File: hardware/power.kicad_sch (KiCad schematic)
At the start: 48 parts, among them J1 USB4085-GF-A, J2 Batteries, J3 Conn_01x02, J4 Conn_01x02, J5 Conn_01x02, J6 Conn_01x02, Q1 PMOS, Q2 PMOS, Q3 PMOS, U1 USBLC6-2SC6, U2 TLV76733DGNR

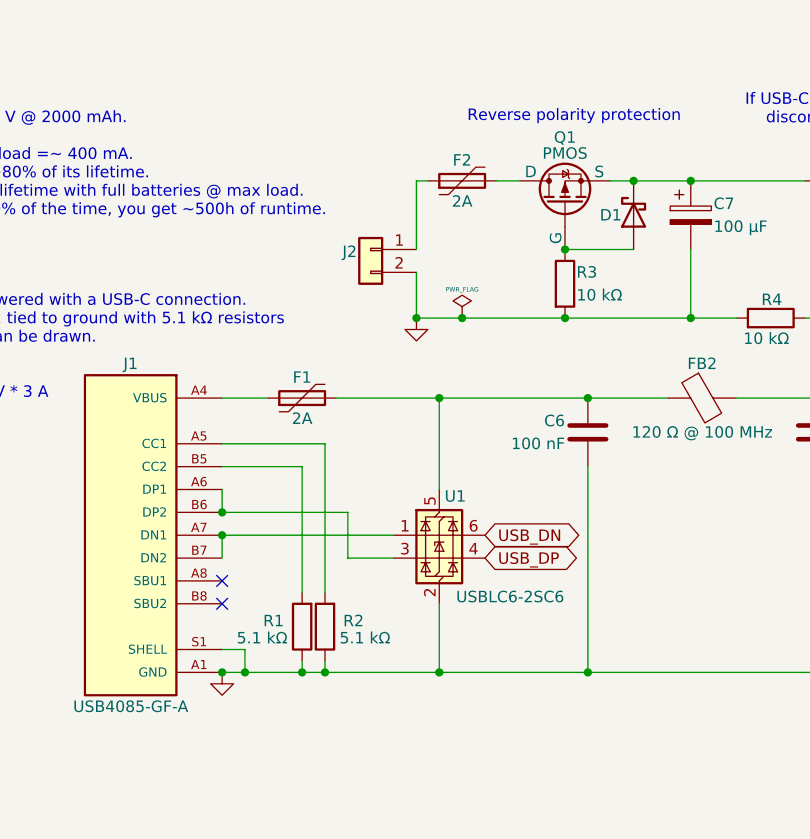
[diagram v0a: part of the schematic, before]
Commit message: HW: Layout power section
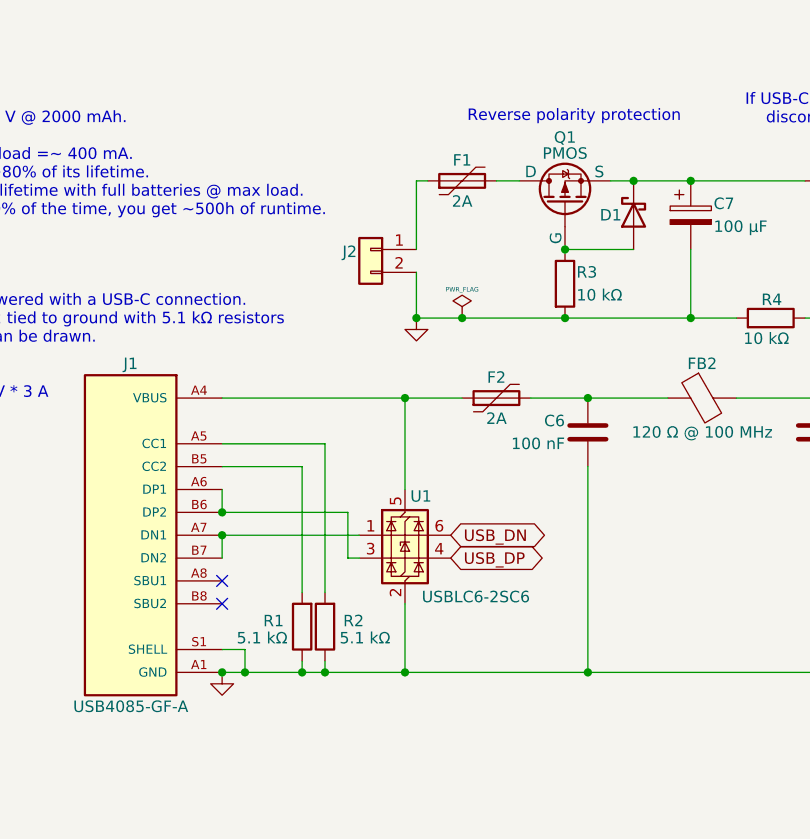
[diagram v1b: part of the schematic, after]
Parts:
- renumbered F2 to F1, F1 to F2
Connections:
- net at F2.1, J1.A4 (VBUS), J1.A9 (VBUS)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: now also U1.5 (VBUS)
- net at C6.1, F2.2, FB2.1: no longer U1.5 (VBUS)
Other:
- moved on the sheet: F2, U1
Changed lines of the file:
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@@
 	)
 	(junction
+		(at 116.84 66.04)
+		(diameter 0)
+		(color 0 0 0 0)
+	)
+	(junction
 		(at 116.84 96.52)
 		(diameter 0)
@@
 	)
 	(junction
-		(at 116.84 66.04)
+		(at 96.52 66.04)
 		(diameter 0)
 		(color 0 0 0 0)
@@
 	)
 	(junction
-		(at 100.33 66.04)
-		(diameter 0)
-		(color 0 0 0 0)
-	)
-	(junction
 		(at 170.18 88.9)
 		(diameter 0)
@@
 	)
 	(junction
-		(at 100.33 96.52)
-		(diameter 0)
-		(color 0 0 0 0)
-	)
-	(junction
 		(at 91.44 185.42)
 		(diameter 0)
@@
 	)
 	(junction
+		(at 96.52 96.52)
+		(diameter 0)
+		(color 0 0 0 0)
+	)
+	(junction
 		(at 204.47 148.59)
 		(diameter 0)
@@
 	(wire
 		(pts
-			(xy 100.33 66.04) (xy 100.33 76.2)
+			(xy 96.52 66.04) (xy 96.52 76.2)
 		)
 		(stroke
@@
 	(wire
 		(pts
-			(xy 100.33 66.04) (xy 116.84 66.04)
+			(xy 229.87 41.91) (xy 231.14 41.91)
 		)
 		(stroke
@@
 	(wire
 		(pts
-			(xy 229.87 41.91) (xy 231.14 41.91)
+			(xy 80.01 193.04) (xy 91.44 193.04)
 		)
 		(stroke
@@
 	(wire
 		(pts
-			(xy 80.01 193.04) (xy 91.44 193.04)
+			(xy 78.74 96.52) (xy 85.09 96.52)
 		)
 		(stroke
@@
 	(wire
 		(pts
-			(xy 78.74 96.52) (xy 85.09 96.52)
+			(xy 163.83 148.59) (xy 172.72 148.59)
 		)
 		(stroke
@@
 	(wire
 		(pts
-			(xy 163.83 148.59) (xy 172.72 148.59)
+			(xy 68.58 185.42) (xy 80.01 185.42)
 		)
 		(stroke
@@
 	(wire
 		(pts
-			(xy 68.58 185.42) (xy 80.01 185.42)
+			(xy 96.52 66.04) (xy 102.87 66.04)
 		)
 		(stroke
@@
 	(wire
 		(pts
-			(xy 100.33 96.52) (xy 116.84 96.52)
+			(xy 146.05 49.53) (xy 146.05 57.15)
 		)
 		(stroke
@@
 	(wire
 		(pts
-			(xy 146.05 49.53) (xy 146.05 57.15)
+			(xy 96.52 96.52) (xy 116.84 96.52)
 		)
 		(stroke
@@
 	(wire
 		(pts
-			(xy 88.9 66.04) (xy 100.33 66.04)
+			(xy 229.87 66.04) (xy 238.76 66.04)
 		)
 		(stroke
@@
 	(wire
 		(pts
-			(xy 229.87 66.04) (xy 238.76 66.04)
+			(xy 194.31 130.81) (xy 207.01 130.81)
 		)
 		(stroke
@@
 	(wire
 		(pts
-			(xy 194.31 130.81) (xy 207.01 130.81)
+			(xy 76.2 81.28) (xy 91.44 81.28)
 		)
 		(stroke
@@
 	(wire
 		(pts
-			(xy 76.2 81.28) (xy 95.25 81.28)
+			(xy 128.27 57.15) (xy 133.35 57.15)
 		)
 		(stroke
@@
 	(wire
 		(pts
-			(xy 128.27 57.15) (xy 133.35 57.15)
+			(xy 168.91 123.19) (xy 181.61 123.19)
 		)
 		(stroke
@@
 	(wire
 		(pts
-			(xy 168.91 123.19) (xy 181.61 123.19)
+			(xy 182.88 96.52) (xy 191.77 96.52)
 		)
 		(stroke
@@
 	(wire
 		(pts
-			(xy 182.88 96.52) (xy 191.77 96.52)
+			(xy 102.87 57.15) (xy 114.3 57.15)
 		)
 		(stroke
@@
 	(wire
 		(pts
-			(xy 102.87 57.15) (xy 114.3 57.15)
+			(xy 96.52 88.9) (xy 96.52 96.52)
 		)
 		(stroke
@@
 	(wire
 		(pts
-			(xy 100.33 88.9) (xy 100.33 96.52)
+			(xy 110.49 66.04) (xy 116.84 66.04)
 		)
 		(stroke
@@
 	(wire
 		(pts
-			(xy 90.17 83.82) (xy 95.25 83.82)
+			(xy 90.17 83.82) (xy 91.44 83.82)
 		)
 		(stroke
@@
 	(wire
 		(pts
-			(xy 87.63 96.52) (xy 100.33 96.52)
+			(xy 87.63 96.52) (xy 96.52 96.52)
 		)
 		(stroke
@@
 	(wire
 		(pts
-			(xy 81.28 66.04) (xy 76.2 66.04)
+			(xy 76.2 66.04) (xy 96.52 66.04)
 		)
 		(stroke
@@
 	(global_label "USB_DP"
 		(shape bidirectional)
-		(at 105.41 83.82 0)
+		(at 101.6 83.82 0)
 		(fields_autoplaced yes)
 		(effects
@@
 		)
 		(property "Intersheetrefs" "${INTERSHEET_REFS}"
-			(at 116.0111 83.82 0)
+			(at 112.2011 83.82 0)
 			(effects
 				(font
@@
 	(global_label "USB_DN"
 		(shape bidirectional)
-		(at 105.41 81.28 0)
+		(at 101.6 81.28 0)
 		(fields_autoplaced yes)
 		(effects
@@
 		)
 		(property "Intersheetrefs" "${INTERSHEET_REFS}"
-			(at 116.0716 81.28 0)
+			(at 112.2616 81.28 0)
 			(effects
 				(font
@@
 	(symbol
 		(lib_id "Device:Polyfuse")
-		(at 85.09 66.04 90)
+		(at 106.68 66.04 90)
 		(unit 1)
 		(exclude_from_sim no)
@@
 		(on_board yes)
 		(dnp no)
-		(property "Reference" "F1"
-			(at 85.09 63.754 90)
+		(property "Reference" "F2"
+			(at 106.68 63.754 90)
 			(effects
 				(font
@@
 		)
 		(property "Value" "2A"
-			(at 85.09 68.326 90)
+			(at 106.68 68.326 90)
 			(effects
 				(font
@@
 		)
 		(property "Footprint" "Fuse:Fuse_0805_2012Metric"
-			(at 90.17 64.77 0)
+			(at 111.76 64.77 0)
 			(effects
 				(font
@@
 		)
 		(property "Datasheet" "~"
-			(at 85.09 66.04 0)
+			(at 106.68 66.04 0)
 			(effects
 				(font
@@
 		)
 		(property "Description" "Resettable fuse, polymeric positive temperature coefficient"
-			(at 85.09 66.04 0)
+			(at 106.68 66.04 0)
 			(effects
 				(font
@@
 		)
 		(property "Digi-Key Part Number" "13-SMD0805B110TFCT-ND"
-			(at 85.09 66.04 0)
+			(at 106.68 66.04 0)
 			(effects
 				(font
@@
 		)
 		(property "Manufacturer" "YAGEO"
-			(at 85.09 66.04 0)
+			(at 106.68 66.04 0)
 			(effects
 				(font
@@
 		)
 		(property "Manufacturer Part Number" "SMD0805B110TF"
-			(at 85.09 66.04 0)
+			(at 106.68 66.04 0)
 			(effects
 				(font
@@
 			(project "iida_devkit"
 				(path "/b12a6e25-97fb-4aba-bc96-af8db389bb9a/8a51e004-740e-440f-9bfb-b035bcbeb0d2"
-					(reference "F1")
+					(reference "F2")
 					(unit 1)
 				)
@@
 		(on_board yes)
 		(dnp no)
-		(property "Reference" "F2"
+		(property "Reference" "F1"
 			(at 102.87 39.624 90)
 			(effects
@@
 			(project "iida_devkit"
 				(path "/b12a6e25-97fb-4aba-bc96-af8db389bb9a/8a51e004-740e-440f-9bfb-b035bcbeb0d2"
-					(reference "F2")
+					(reference "F1")
 					(unit 1)
 				)
@@
 	(symbol
 		(lib_id "Power_Protection:USBLC6-2SC6")
-		(at 100.33 81.28 0)
+		(at 96.52 81.28 0)
 		(unit 1)
 		(exclude_from_sim no)
@@
 		(dnp no)
 		(property "Reference" "U1"
-			(at 102.108 76.962 0)
+			(at 98.298 76.962 0)
 			(effects
 				(font
@@
 		)
 		(property "Value" "USBLC6-2SC6"
-			(at 108.204 88.138 0)
+			(at 104.394 88.138 0)
 			(effects
 				(font
@@
 		)
 		(property "Footprint" "Package_TO_SOT_SMD:SOT-23-6"
-			(at 100.33 93.98 0)
+			(at 96.52 93.98 0)
 			(effects
 				(font
@@
 		)
 		(property "Datasheet" "https://www.st.com/resource/en/datasheet/usblc6-2.pdf"
-			(at 105.41 72.39 0)
+			(at 101.6 72.39 0)
 			(effects
 				(font
@@
 		)
 		(property "Description" "Very low capacitance ESD protection diode, 2 data-line, SOT-23-6"
-			(at 100.33 81.28 0)
+			(at 96.52 81.28 0)
 			(effects
 				(font
@@
 		)
 		(property "Manufacturer" "STMicroelectronics"
-			(at 100.33 81.28 90)
+			(at 96.52 81.28 90)
 			(effects
 				(font
@@
 		)
 		(property "Manufacturer Part Number" "USBLC6-2SC6"
-			(at 100.33 81.28 90)
+			(at 96.52 81.28 90)
 			(effects
 				(font
@@
 		)
 		(property "Digi-Key Part Number" "497-5235-1-ND"
-			(at 100.33 81.28 90)
+			(at 96.52 81.28 90)
 			(effects
 				(font
